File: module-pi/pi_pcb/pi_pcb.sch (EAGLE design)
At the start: 8 parts, among them IC3 PIC16F870SO, K1 PIN20X2

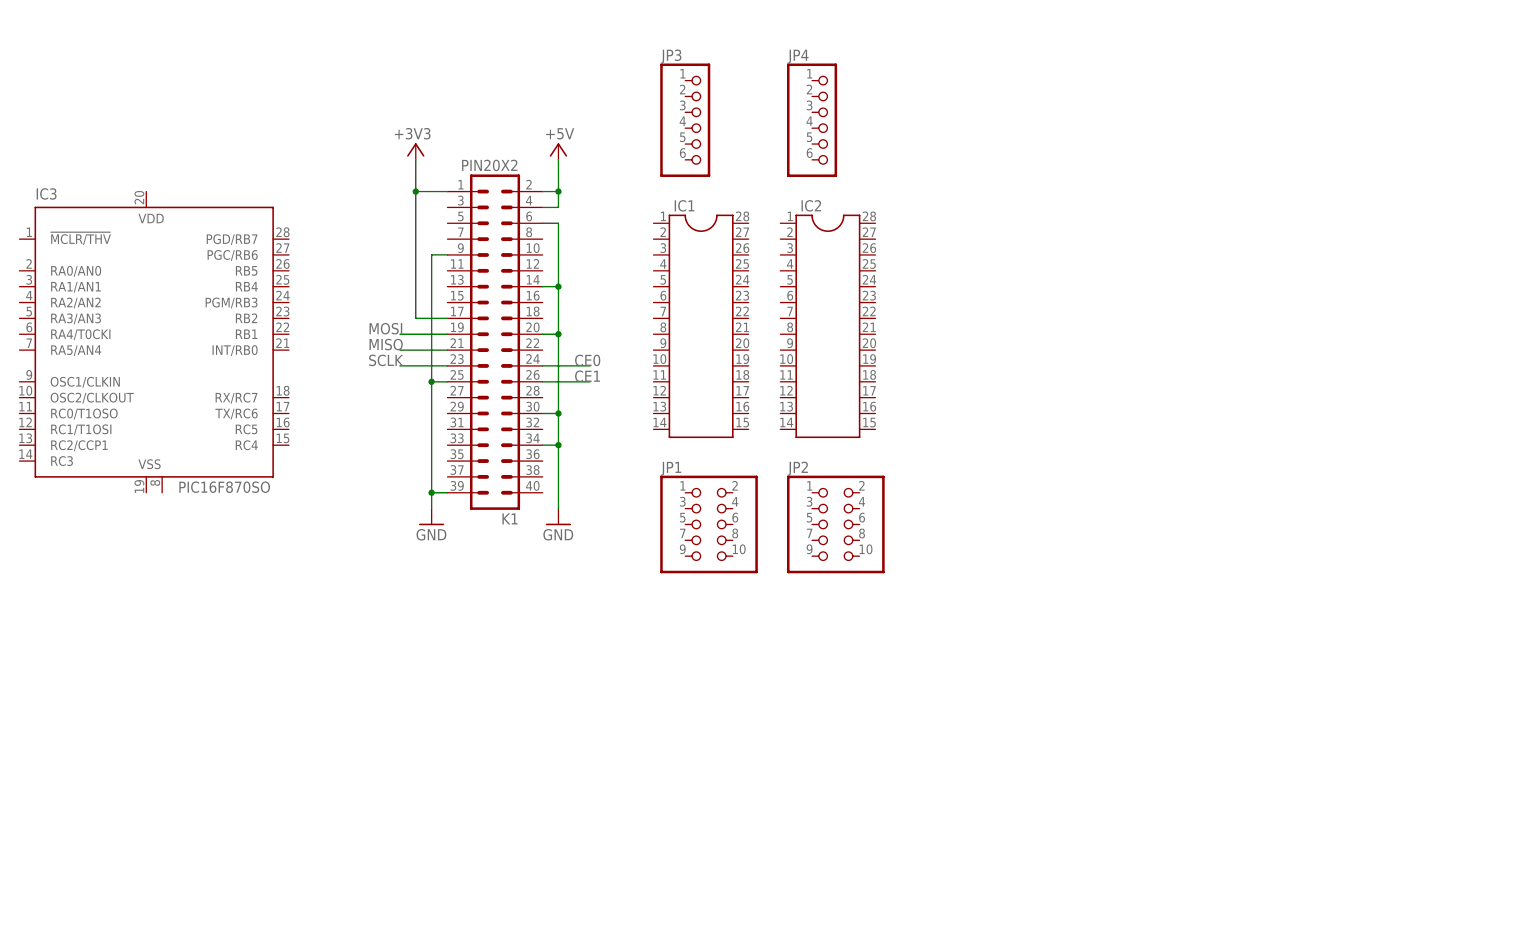
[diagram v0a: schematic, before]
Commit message: First pi hat PCB submitted.
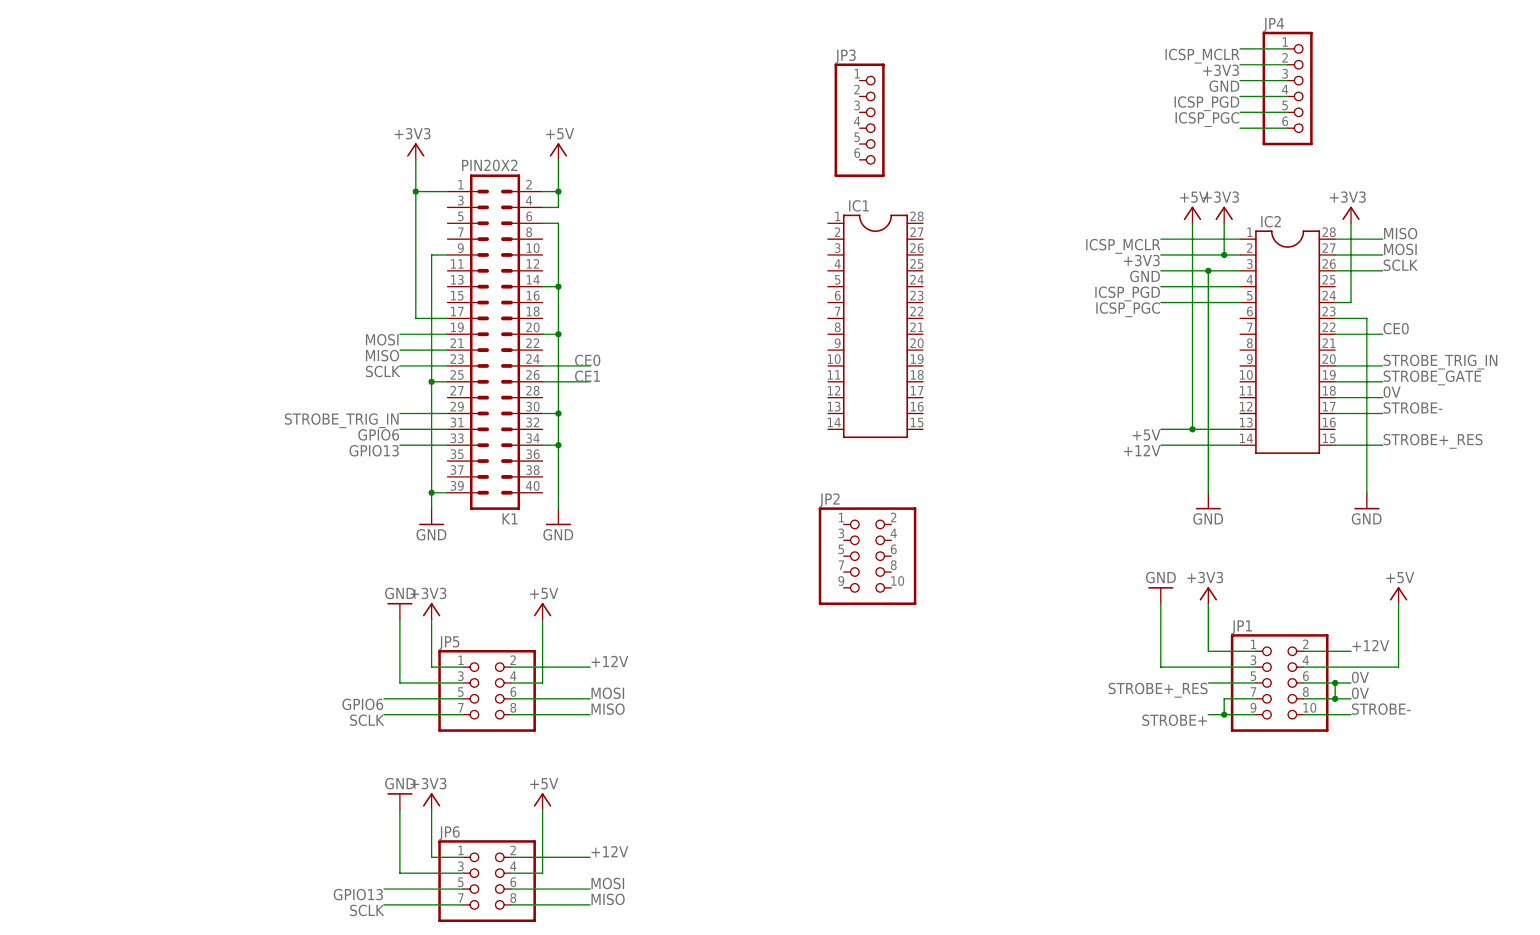
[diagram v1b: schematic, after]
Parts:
- removed IC3: PIC16F870SO, microchip:PIC16F870SO
- added JP5, JP6: (no value), pinhead:PINHD-2X4
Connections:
- new net +12V: IC2.14, JP1.2, JP5.2, JP6.2
- new net 0V: IC2.18, JP1.6, JP1.8
- new net GPIO13: JP6.5, K1.33
- new net GPIO6: JP5.5, K1.31
- new net ICSP_MCLR: IC2.1, JP4.1
- new net ICSP_PGC: IC2.5, JP4.5
- new net ICSP_PGD: IC2.4, JP4.4
- new net N$6: JP4.6
- new net STROBE+: JP1.7, JP1.9
- new net STROBE+_RES: IC2.15, JP1.5
- new net STROBE-: IC2.17, JP1.10
- new net STROBE_GATE: IC2.19
- new net STROBE_TRIG_IN: IC2.20, K1.29
- net +3V3: now also IC2.2, IC2.24, JP1.1, JP4.2, JP5.1, JP6.1
- net +5V: now also IC2.13, JP1.4, JP5.4, JP6.4
- net CE0: now also IC2.22
- net GND: now also IC2.23, IC2.3, JP1.3, JP4.3, JP5.3, JP6.3
- net MISO: now also IC2.28, JP5.8, JP6.8
- net MOSI: now also IC2.27, JP5.6, JP6.6
- net SCLK: now also IC2.26, JP5.7, JP6.7
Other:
- moved on the sheet: IC1, IC2, JP1, JP2, JP3, JP4
